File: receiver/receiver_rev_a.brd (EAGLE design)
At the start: 100 x 80 mm, 1 part

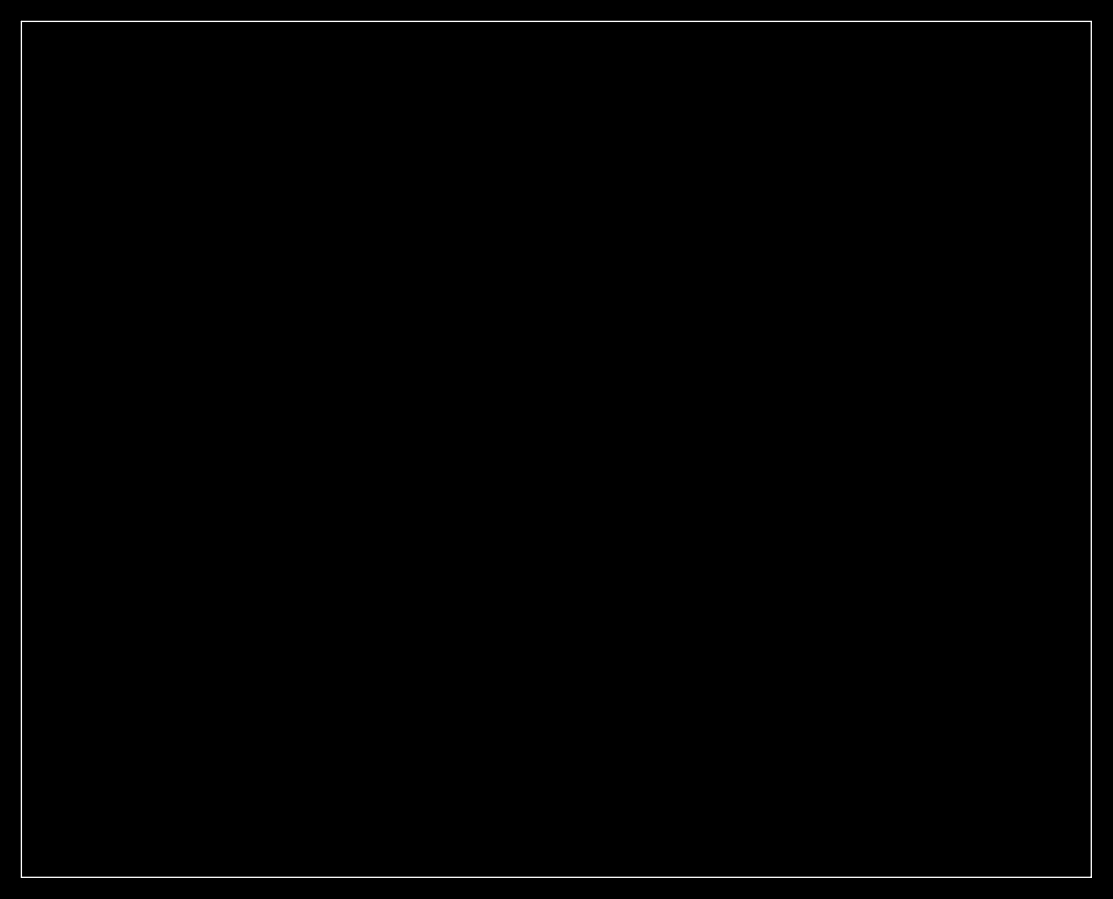
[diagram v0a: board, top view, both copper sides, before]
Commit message: Mostly done with the receiver
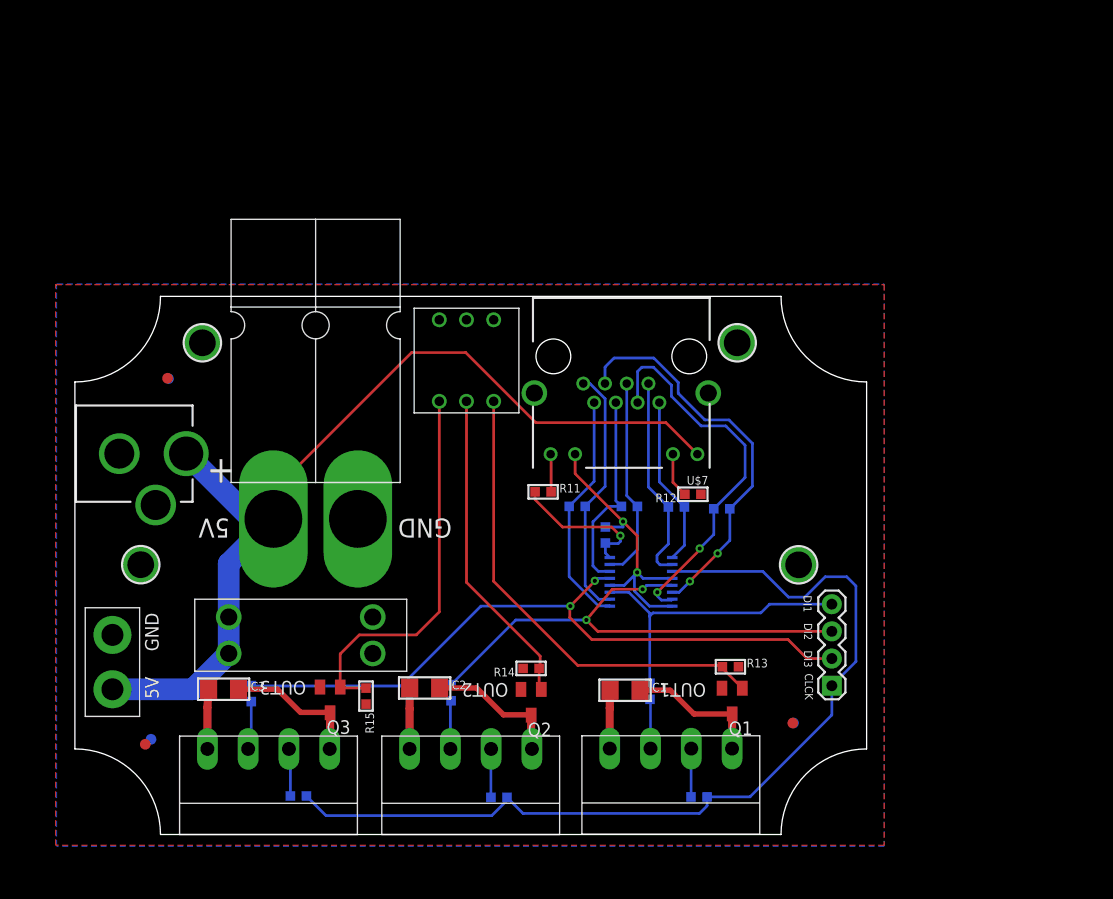
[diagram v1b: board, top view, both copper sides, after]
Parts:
- added C1, C2, C3: 100uF, microbuilder:1206
- added C4: 0.1uF, microbuilder:0603-MINI
- added CN1: (no value), microbuilder:DCJACK_2MM_PTH
- added FID1, FID2, FID3, FID4, FID5, FID6: FIDUCIAL, adafruit:FIDUCIAL_1MM
- added FUSE: (no value), Custom:FUSE-HOLDER-3557
- added J1: POWERPOLE_POWER45A_HORIZONTAL_DRILL, powerpoles:POWERPOLE_PAIR_45A_HORIZ_HOLE
- added JP1: (no value), SparkFun-Connectors:1X04
- added JP2: (no value), SparkFun-Connectors:1X02_XTRA_BIG
- added OUT1, OUT2, OUT3: MC4, con-phoenix-381_l:MC4
- added Q1, Q2, Q3: (no value), Custom:SC59
- added R1, R10, R2, R3, R4, R5, R6, R7, R8, R9: 120, microbuilder:0603-MINI
- added R11, R12: 220, microbuilder:0603-MINI
- added R13, R14, R15: 10k, microbuilder:0603-MINI
- added SWITCH: (no value), Custom:194-DIP-SWITCH
- added U$2: (no value), Custom:AK-B-FT21
- added U$3, U$4, U$5, U$6: MOUNTINGHOLE2.5, microbuilder:MOUNTINGHOLE_2.5_PLATED
- added U$7: (no value), Custom:RJHSE-538X
- added U1: (no value), maxim:TSSOP16
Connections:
- new net A+: R1.2, U$7.1, U1.2
- new net A-: R1.1, U$7.2, U1.1
- new net B+: R2.2, U$7.3, U1.14
- new net B-: R2.1, U$7.6, U1.15
- new net C+: R3.2, U$7.4, U1.6
- new net C-: R3.1, U$7.5, U1.7
- new net CLOCK: JP1.1, R6.2, R7.2, R9.2, U1.11
- new net D+: R4.2, U$7.7, U1.10
- new net D-: R4.1, U$7.8, U1.9
- new net DATA1: JP1.4, R5.2, U1.3
- new net DATA2: JP1.3, R8.2, U1.13
- new net DATA3: JP1.2, R10.2, U1.5
- new net GATE1: Q1.G, R13.1, SWITCH.1B
- new net GATE2: Q2.G, R14.1, SWITCH.2B
- new net GATE3: Q3.G, R15.1, SWITCH.3B
- new net GND: C4.2, CN1.GND, J1.BLACK, JP2.2, Q1.S, Q2.S, Q3.S, R11.1, R12.1, R13.2, R14.2, R15.2, U$7.P$1, U$7.P$2, U1.8
- new net GNDBREAK: CN1.GNDBREAK
- new net N$1: OUT1.2, R5.1
- new net N$10: R11.2, U$7.9
- new net N$11: R12.2, U$7.11
- new net N$2: OUT1.3, R6.1
- new net N$3: C1.2, OUT1.4, Q1.D
- new net N$4: OUT2.2, R8.1
- new net N$5: OUT2.3, R7.1
- new net N$6: C2.2, OUT2.4, Q2.D
- new net N$7: OUT3.2, R10.1
- new net N$8: OUT3.3, R9.1
- new net N$9: C3.2, OUT3.4, Q3.D
- new net PREFUSE_VCC: CN1.PWR, FUSE.A1, FUSE.A2, J1.RED, JP2.1, U$7.12
- new net VCC: C1.1, C2.1, C3.1, C4.1, FUSE.B1, FUSE.B2, OUT1.1, OUT2.1, OUT3.1, SWITCH.1A, SWITCH.2A, SWITCH.3A, U$7.10, U1.12, U1.16, U1.4
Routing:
- net PREFUSE_VCC: track 0.00 -> 88.8 mm
- net CLOCK: track 0.00 -> 88.0 mm
- net DATA3: track 0.00 -> 64.9 mm, vias 0 -> 2
- net DATA2: track 0.00 -> 48.0 mm, vias 0 -> 2
- net VCC: track 0.00 -> 44.9 mm, vias 0 -> 2
- net GATE1: track 0.00 -> 44.3 mm
- net B+: track 0.00 -> 37.0 mm, vias 0 -> 2
- net GATE3: track 0.00 -> 36.2 mm
- net B-: track 0.00 -> 35.8 mm, vias 0 -> 2
- net GATE2: track 0.00 -> 29.9 mm
- net DATA1: track 0.00 -> 28.6 mm
- net A+: track 0.00 -> 23.7 mm
- net A-: track 0.00 -> 22.2 mm
- net D+: track 0.00 -> 19.4 mm
- net C-: track 0.00 -> 19.1 mm
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- added copper zone on layer 1, net GND
- added copper zone on layer 16, net VCC
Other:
- board size 100 x 80 mm -> 74 x 50.3 mm
- board text added: "5V"
- board text added: "CLCK"
- board text added: "DI1"
- board text added: "DI2"
- board text added: "DI3"
- board text added: "GND"
